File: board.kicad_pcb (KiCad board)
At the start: 2 copper layers, 35 x 40 mm, 24 parts, among them J1 TEMPS, J2 OLED, J3 RELAY, J4 RELAY_EN, J5 USB_B_Micro, Q1 BC847, Q2 BC847, U1 ESP32-WROOM-32, U2 AMS1117-3.3, U3 CP2104

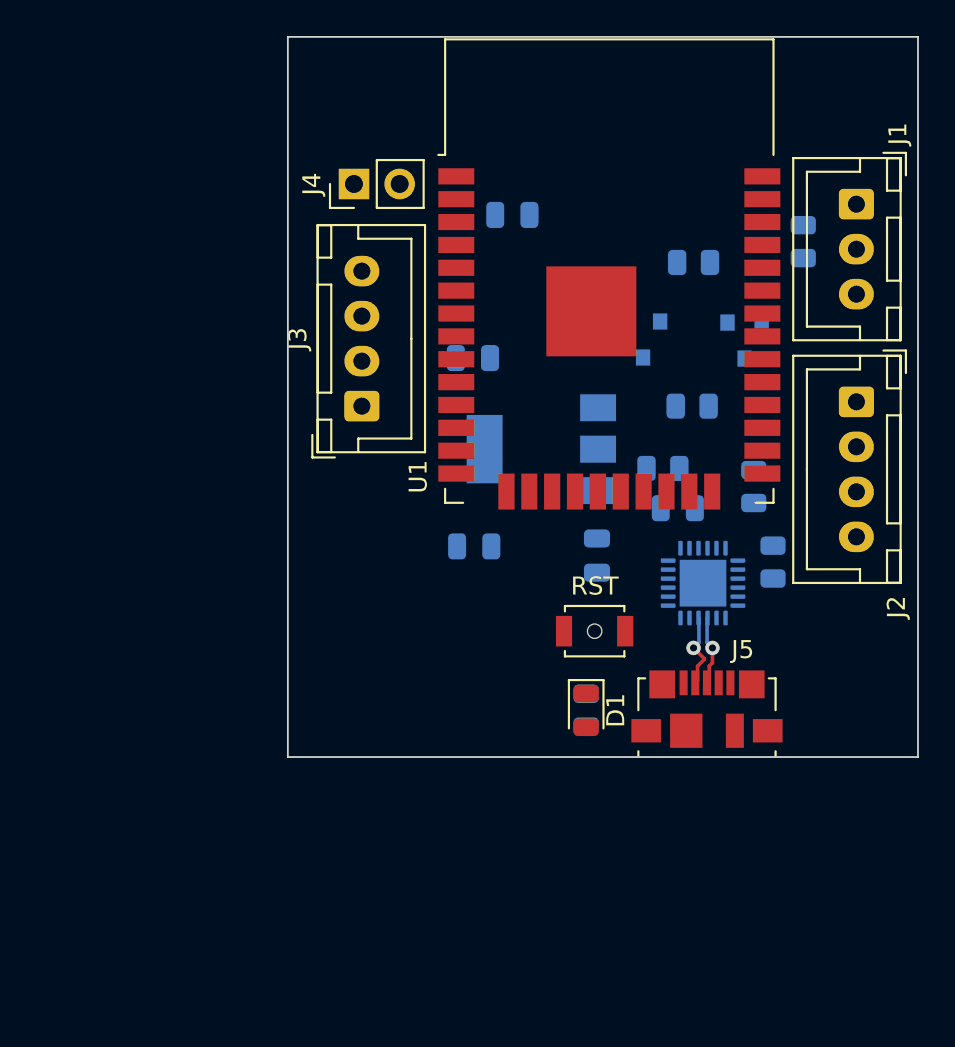
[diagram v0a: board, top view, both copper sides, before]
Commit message: with programmer
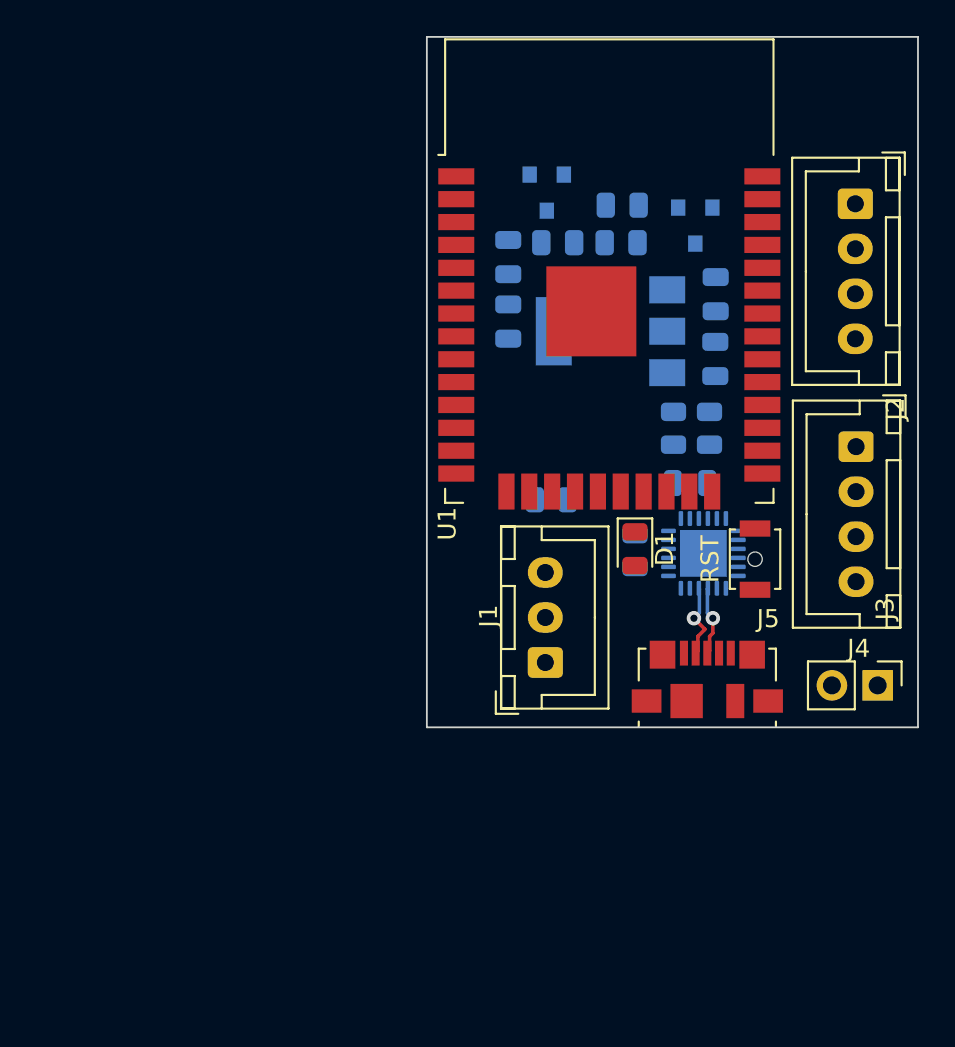
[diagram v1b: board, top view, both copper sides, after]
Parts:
- moved J4 40.3 mm to (152.8, 123.0), turned to 270 degrees
- moved J1 30.8 mm to (134.3, 121.8), turned to 90 degrees
- moved J3 27.5 mm to (151.6, 109.8), turned to 270 degrees
- moved R1 20.0 mm to (134.6, 112.7), turned to 180 degrees
- moved C5 19.4 mm to (143.8, 101.3), turned to 90 degrees
- moved R3 13.8 mm to (135.0, 98.4), turned to 180 degrees
- moved C1 12.7 mm to (143.7, 104.9), turned to 270 degrees
- moved J2 11.0 mm to (151.5, 96.3)
- moved R6 9.90 mm to (138.5, 98.4)
- moved RST 9.77 mm to (145.9, 116.0), turned to 90 degrees
- moved Q1 9.76 mm to (134.4, 95.7)
- moved D1 9.38 mm to (139.3, 115.4)
- moved R2 9.28 mm to (139.3, 115.5)
- moved R5 8.23 mm to (143.4, 108.7)
- moved U2 7.59 mm to (137.9, 103.3)
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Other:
- board size 35 x 40 mm -> 27.3 x 38.3 mm

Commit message: initial finished board pre-fab
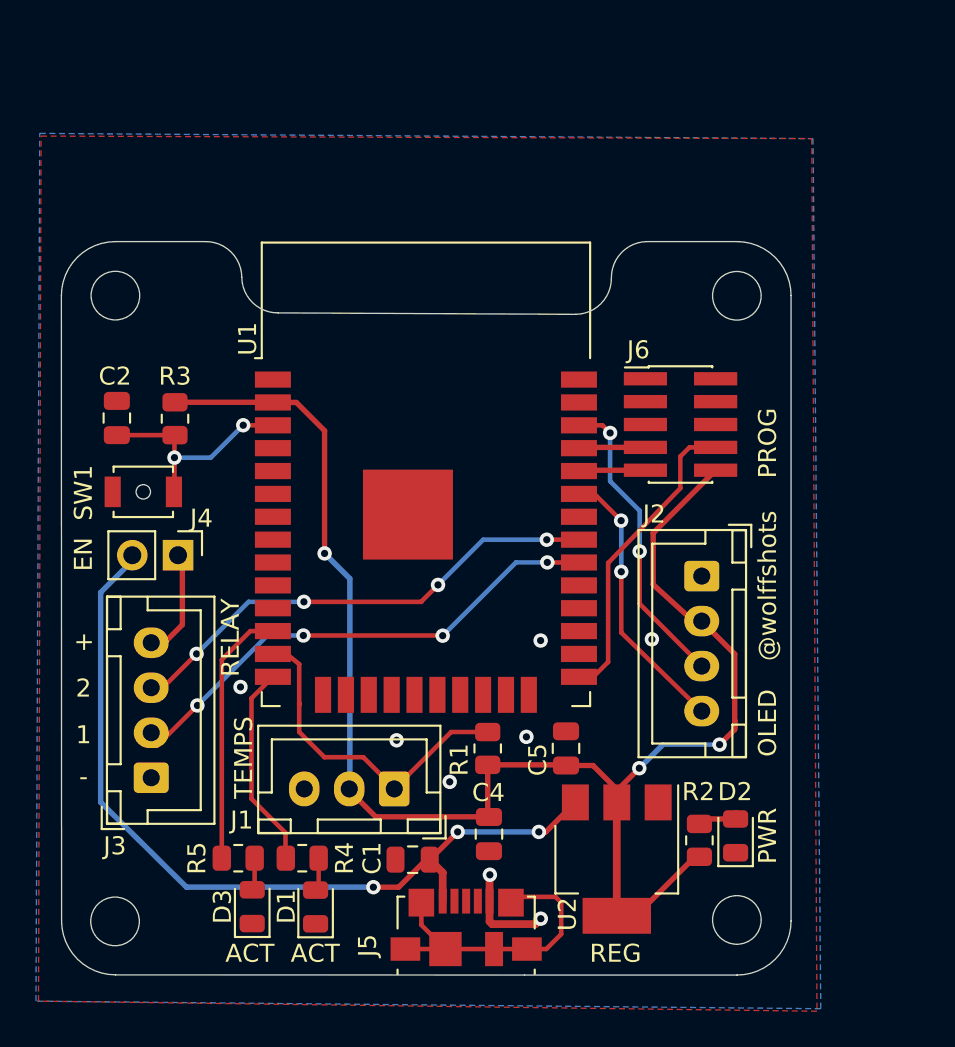
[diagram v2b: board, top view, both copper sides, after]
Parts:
- removed C3: 4.7uF, Capacitor_SMD:C_0805_2012Metric
- removed Q1, Q2: BC847, Package_TO_SOT_SMD:SOT-23
- removed R6, R7: 10K, Resistor_SMD:R_0805_2012Metric
- removed RST: SW_RESET, Button_Switch_SMD:SW_SPST_B3U-1000P-B
- removed U3: CP2104, Package_DFN_QFN:QFN-24-1EP_4x4mm_P0.5mm_EP2.6x2.6mm
- added 1: MH, MountingHole:MountingHole_2.7mm_M2.5, F.Cu at (144.9, 101.4)
- added 2: MH, MountingHole:MountingHole_2.7mm_M2.5, F.Cu at (144.9, 136.1)
- added 3: MH, MountingHole:MountingHole_2.7mm_M2.5, F.Cu at (110.4, 136.1)
- added 4: MH, MountingHole:MountingHole_2.7mm_M2.5, F.Cu at (110.4, 101.4)
- added D2: PLED, LED_SMD:LED_0805_2012Metric, F.Cu at (144.9, 131.4)
- added D3: SLED2, LED_SMD:LED_0805_2012Metric, F.Cu at (118.0, 135.3)
- added G***: LOGO, Graphics:esp32_warm_water, B.Cu at (127.7, 111.5)
- added J6: CONN_PROG, Connector_PinHeader_1.27mm:PinHeader_2x05_P1.27mm_Vertical_SMD, F.Cu at (141.8, 108.5)
- added SW1: SW_RESET, Button_Switch_SMD:SW_SPST_B3U-1000P-B, F.Cu at (112.0, 112.3)
- C1, C2, C4, C5, R1, R3, U2: moved to F.Cu
- D1: value LED -> SLED1
- R2: value R -> 330; moved to F.Cu
- R4, R5: value 470 -> 330; moved to F.Cu
- moved J3 43.3 mm to (112.4, 128.2), turned to 90 degrees
- moved J4 39.5 mm to (113.9, 115.8)
- moved R5 35.4 mm to (117.2, 132.6), turned to 0 degrees
- moved C1 32.5 mm to (126.9, 132.7), turned to 0 degrees
- moved R4 31.6 mm to (120.8, 132.6), turned to 0 degrees
- moved U2 29.3 mm to (138.3, 132.7), turned to 270 degrees
- moved C4 28.5 mm to (131.2, 131.3), turned to 90 degrees
- moved D1 26.7 mm to (121.5, 135.3), turned to 90 degrees
- moved C5 26.6 mm to (135.4, 126.5)
- moved C2 23.5 mm to (110.5, 108.2), turned to 270 degrees
- moved R3 23.4 mm to (113.7, 108.2), turned to 270 degrees
- moved J2 22.4 mm to (143.0, 117.0)
- moved J5 19.2 mm to (129.9, 136.5)
- moved R2 16.5 mm to (142.9, 131.6), turned to 90 degrees
- moved U1 15.2 mm to (127.7, 114.3)
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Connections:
- net Net-(J5-Pad4) renamed /USB_4
- net Net-(J5-Pad6) renamed /USB_6
- net Net-(U1-Pad10) renamed /IO25
- net Net-(U1-Pad11) renamed /IO26
- net Net-(U1-Pad16) renamed /IO13
- net Net-(U1-Pad17) renamed /SD2
- net Net-(U1-Pad18) renamed /SD3
- net Net-(U1-Pad19) renamed /CMD
- net Net-(U1-Pad20) renamed /CLK
- net Net-(U1-Pad21) renamed /SD0
- net Net-(U1-Pad22) renamed /SD1
- net Net-(U1-Pad23) renamed /IO15
- net Net-(U1-Pad24) renamed /IO2
- net Net-(U1-Pad26) renamed /IO4
- net Net-(U1-Pad27) renamed /IO16
- net Net-(U1-Pad28) renamed /IO17
- net Net-(U1-Pad29) renamed /IO5
- net Net-(U1-Pad37) renamed /IO23
- net Net-(U1-Pad6) renamed /IO34
- net Net-(U1-Pad7) renamed /IO35
- net Net-(U1-Pad8) renamed /IO32
- net Net-(U1-Pad9) renamed /IO33
- net RESET renamed /RESET
- D1 pad 2: /LED_V -> /SLED_V1
- J5 pad 2: D- -> /USB_2
- J5 pad 3: D+ -> /USB_3
- R2 pad 2: /LED_V -> /PLED_V
- R4 pad 1: RX_CP -> SLED1
- R4 pad 2: /TX_ESP -> /SLED_V1
- R5 pad 1: /RX_ESP -> SLED2
- R5 pad 2: TX_CP -> /SLED_V2
- U1 pad 12: Net-(U1-Pad12) -> SLED2
- U1 pad 14: Net-(U1-Pad14) -> SLED1
- U1 pad 34: /RX_ESP -> RX
- U1 pad 35: /TX_ESP -> TX
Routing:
- net +3V3: track 0.00 -> 91.2 mm, vias 0 -> 3
- net VBUS: track 0.00 -> 47.7 mm, vias 0 -> 3
- net CH1: track 0.00 -> 28.7 mm, vias 0 -> 4
- net CH2: track 0.00 -> 27.5 mm, vias 0 -> 4
- net GPIO14: track 0.00 -> 18.7 mm
- net /USB_6: track 0.00 -> 17.5 mm
- net GPIO0: track 0.00 -> 17.2 mm
- net SCL: track 0.00 -> 17.0 mm, vias 0 -> 2
- net SDA: track 0.00 -> 16.2 mm, vias 0 -> 2
- net SLED2: track 0.00 -> 14.5 mm
- net /RESET: track 0.00 -> 12.7 mm, vias 0 -> 2
- net SLED1: track 0.00 -> 11.4 mm
- net /RELAY_V: track 0.00 -> 6.22 mm
- net GND: track 0.00 -> 5.64 mm, vias 0 -> 8
- net D-: track 4.19 -> 0.00 mm, vias 1 -> 0
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- added copper zone on B.Cu, net GND
- added copper zone on F.Cu, net GND
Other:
- board size 27.3 x 38.3 mm -> 40.5 x 40.7 mm
- board text added: "@wolffshots"
- board text added: "JLCJLCJLCJLC"
